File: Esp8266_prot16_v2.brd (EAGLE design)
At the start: 54.7 x 34.2 mm, 22 parts, among them IC2 TPS77033, X1 22-23-2031

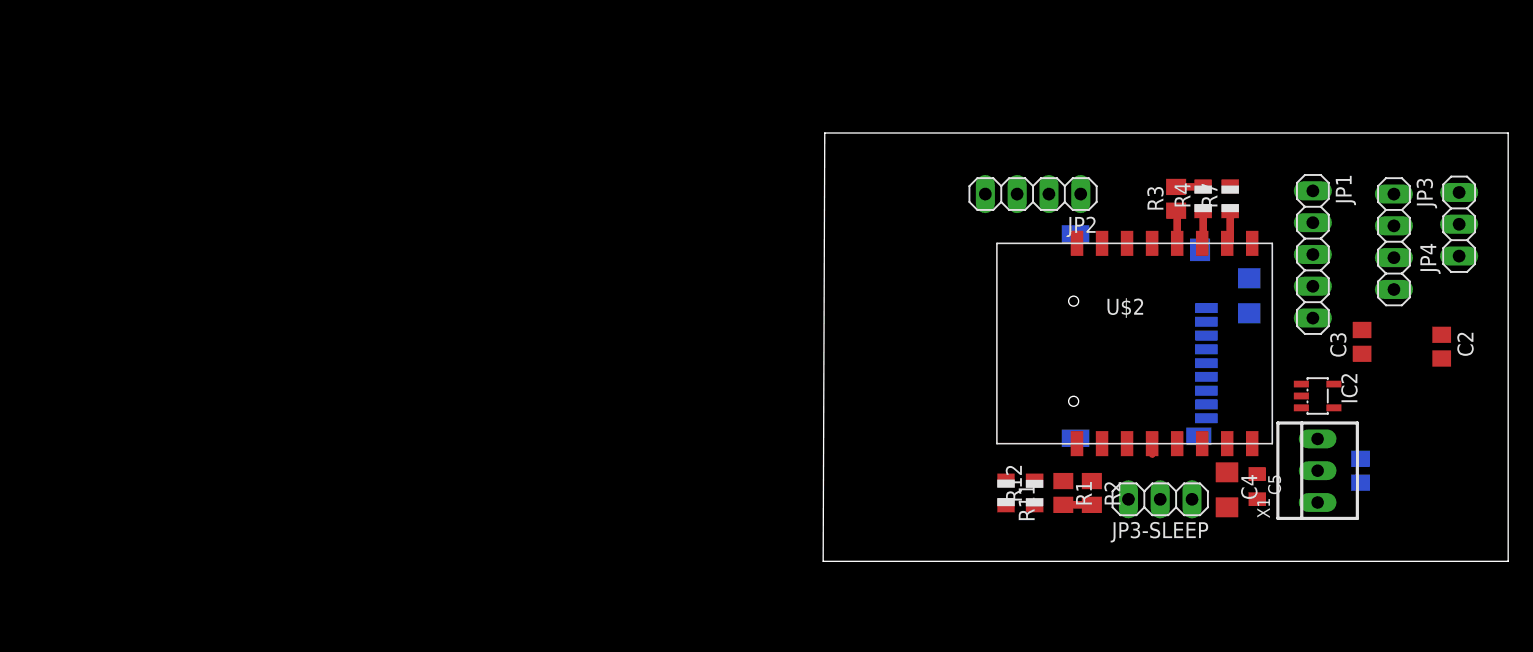
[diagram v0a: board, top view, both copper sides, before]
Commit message: Inicio Repositorio
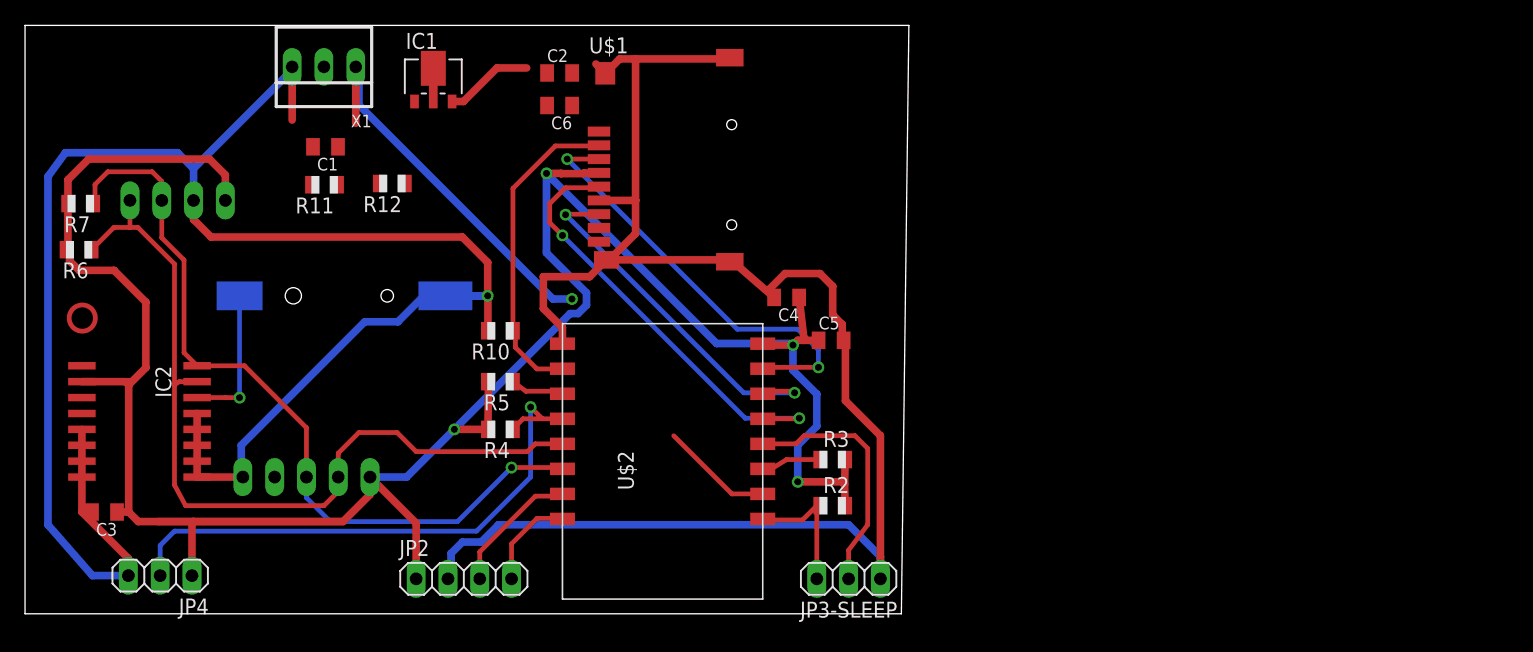
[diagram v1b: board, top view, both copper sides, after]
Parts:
- removed R1: 10K, adafruit:M0805
- added IC1: (no value), v-reg:SOT89R
- added R10, R5: 10K, adafruit:R0805
- added R6: 3K9, adafruit:R0805
- added U$3: CH291-1220LF, battery:CH291-1220LF
- C1, C2: value 0.1uF -> (none); device rcl:C0805 -> adafruit:C0805K
- C3: value 2.2uF -> (none); device rcl:C0805 -> adafruit:C0805K
- C4, C6: device adafruit:C1206 -> adafruit:C0805K
- IC2: value TPS77033 -> DS3231/SO; device texas:SOT23-DBV -> adafruit:SO16W
- JP1: device pinhead:1X05 -> pinhead:1X05/90
- JP3: device pinhead:1X04 -> pinhead:1X04/90
- R2, R3: device adafruit:M0805 -> adafruit:R0805
- R7: value 10K -> 3K9
- moved JP4 107.5 mm to (10.8, 3.05), turned to 180 degrees
- moved C3 101.4 mm to (6.35, 8.13), turned to 180 degrees
- moved JP3 97.4 mm to (12.2, 36.8), flipped to the bottom, turned to 0 degrees
- moved IC2 94.1 mm to (9.14, 15.4)
- moved R7 91.8 mm to (4.45, 32.8), turned to 180 degrees
- moved C1 86.6 mm to (24.0, 37.3), flipped to the top, turned to 180 degrees
- moved X1 85.7 mm to (23.9, 43.7), turned to 180 degrees
- moved JP1 83.2 mm to (22.5, 7.11), flipped to the bottom, turned to 180 degrees
- moved C2 73.8 mm to (42.7, 43.2), turned to 0 degrees
- moved R11 59.7 mm to (23.9, 34.3), turned to 180 degrees
- moved R4 59.1 mm to (38.0, 14.7), turned to 180 degrees
- moved C6 57.1 mm to (42.7, 40.6), flipped to the top, turned to 180 degrees
- moved R12 57.0 mm to (29.3, 34.4), turned to 180 degrees
- moved JP2 54.9 mm to (35.1, 2.79), turned to 0 degrees
- moved U$1 50.5 mm to (45.8, 34.7), flipped to the top
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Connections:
- removed net BYPASS: C3.1, IC2.4
- new net BATRTC: IC2.14, U$3.+
- new net NC: JP1.2
- net 3.3V: now also C3.1, IC1.3, IC2.2, JP1.5, R5.2, R6.2, R7.2; no longer IC2.5, JP1.1, R1.2
- net EN: now also R3.1; no longer R2.1
- net GND: now also IC1.1, IC2.10, IC2.11, IC2.12, IC2.13, IC2.5, IC2.6, IC2.7, IC2.8, IC2.9, JP1.1, R10.2, U$3.-; no longer IC2.2, JP1.5, R7.2
- net GPIO0_D3: now also R4.1; no longer R3.1
- net GPIO15_D8: now also R10.1; no longer R7.1
- net GPIO2_D4: now also R5.1; no longer R4.1
- net GPIO4_D2_SDA: now also IC2.15, JP1.4, R6.1; no longer JP1.2
- net GPIO5_D1_SCL: now also IC2.16, R7.1
- net REST: now also R2.1; no longer R1.1
- net RX: now also JP2.3; no longer JP2.4
- net TX: now also JP2.4; no longer JP2.3
- net VBAT: now also IC1.2; no longer IC2.1, IC2.3
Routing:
- net GND: track 0.00 -> 290.5 mm, vias 0 -> 1
- net 3.3V: track 4.82 -> 188.3 mm, vias 0 -> 4
- net GPIO4_D2_SDA: track 0.00 -> 67.6 mm
- net GPIO5_D1_SCL: track 0.00 -> 63.2 mm, vias 0 -> 1
- net GPIO0_D3: track 2.64 -> 47.0 mm, vias 0 -> 1
- net GPIO14_D5: track 0.00 -> 35.4 mm, vias 0 -> 2
- net GPIO13_D7: track 0.00 -> 34.9 mm, vias 0 -> 2
- net VBAT: track 0.00 -> 31.0 mm, vias 0 -> 1
- net GPIO12_D6: track 0.00 -> 29.6 mm, vias 0 -> 2
- net GPIO15_D8: track 2.65 -> 25.6 mm
- net GPIO16_D0: track 1.09 -> 20.0 mm
- net BATRTC: track 0.00 -> 11.5 mm, vias 0 -> 1
- net RX: track 0.00 -> 10.7 mm
- net REST: track 0.30 -> 10.9 mm
- net ADC: track 0.00 -> 9.04 mm
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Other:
- board size 54.7 x 34.2 mm -> 70.6 x 47 mm
